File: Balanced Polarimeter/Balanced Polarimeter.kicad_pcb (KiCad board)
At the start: 2 copper layers, 65 x 46.5 mm, 25 parts, among them IC1 OP27, J1 73100-0105, J2 Conn_01x03_Pin, J3 Conn_01x02_Pin, J5 Conn_01x02_Pin, Q1 MMPQ3904, Q2 MMPQ3904, U1 ADA4898-1YRDZ, U2 ADA4898-1YRDZ

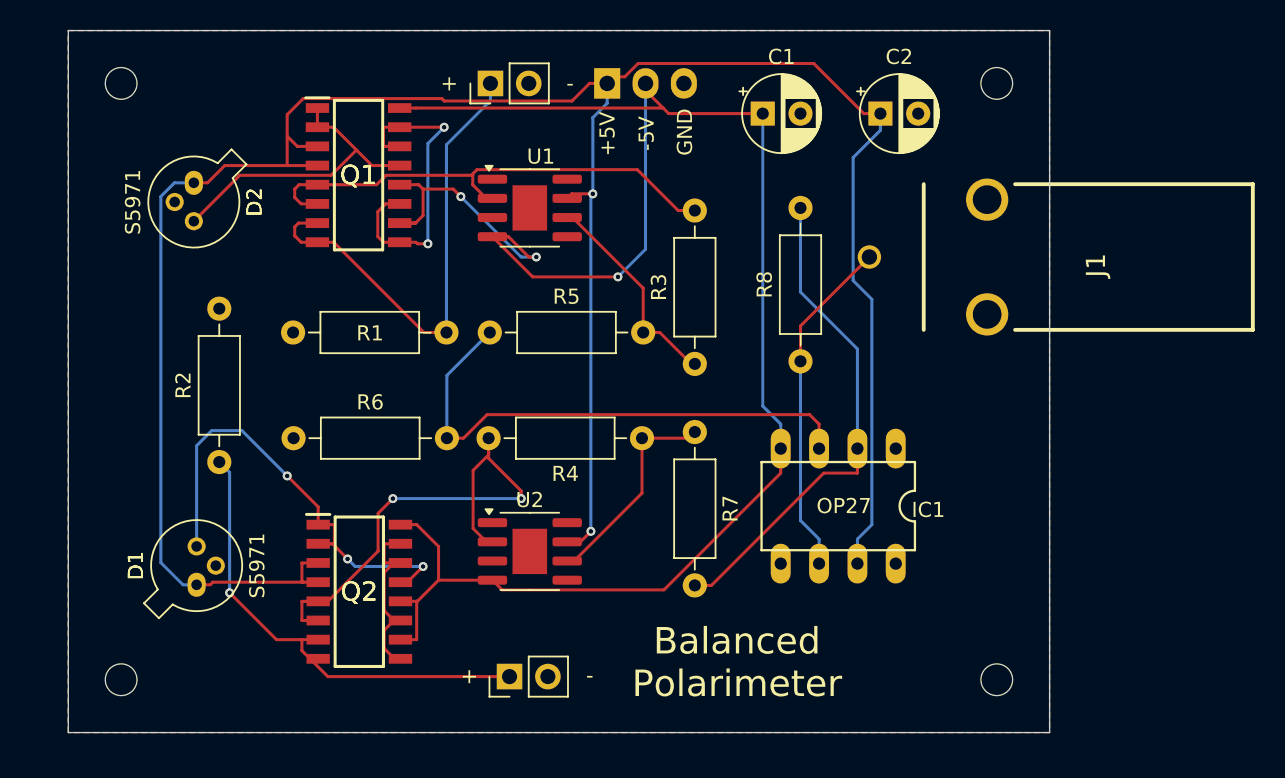
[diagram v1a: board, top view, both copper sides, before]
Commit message: Finalized the PCB Design
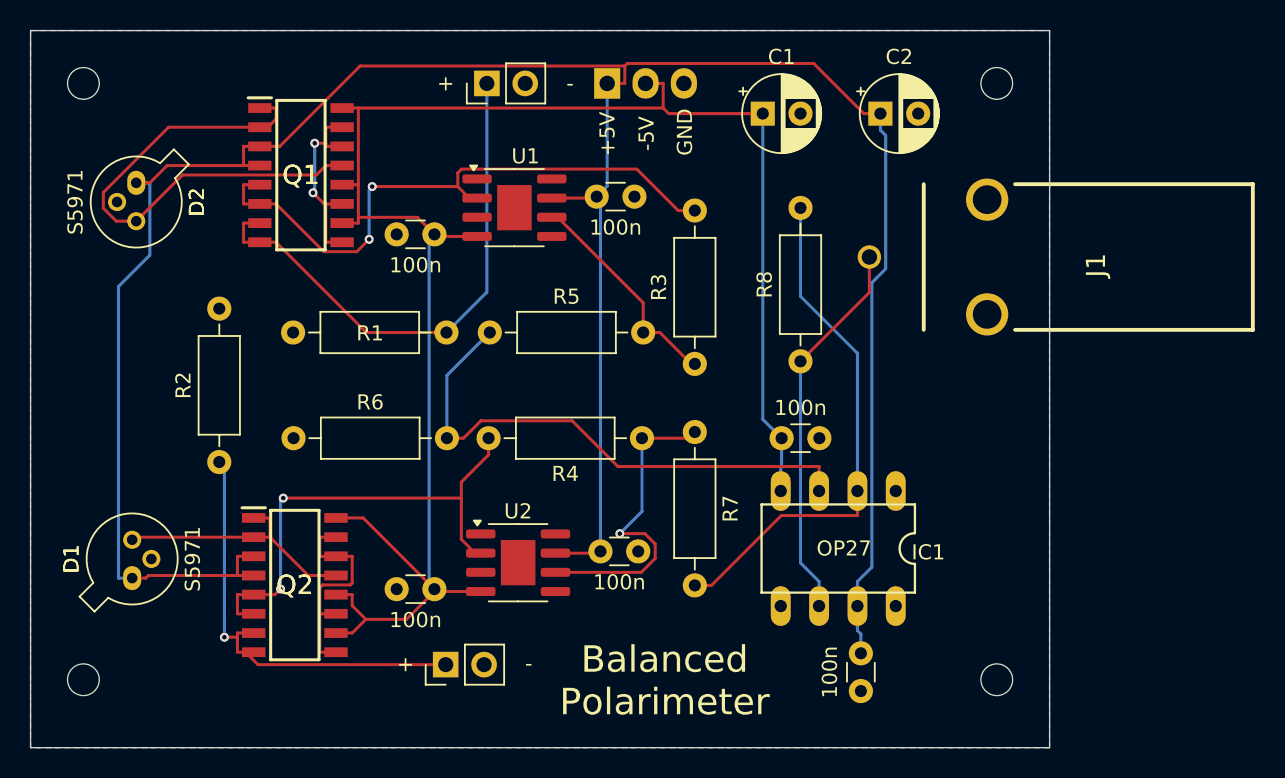
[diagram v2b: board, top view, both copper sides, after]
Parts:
- added C10: 100n, Capacitor_THT:C_Disc_D3.0mm_W1.6mm_P2.50mm, F.Cu at (157.2, 96.0)
- added C11: 100n, Capacitor_THT:C_Disc_D3.0mm_W1.6mm_P2.50mm, F.Cu at (157.0, 72.5)
- added C12: 100n, Capacitor_THT:C_Disc_D3.0mm_W1.6mm_P2.50mm, F.Cu at (143.8, 75.0)
- added C13: 100n, Capacitor_THT:C_Disc_D3.0mm_W1.6mm_P2.50mm, F.Cu at (174.5, 102.8)
- added C14: 100n, Capacitor_THT:C_Disc_D3.0mm_W1.6mm_P2.50mm, F.Cu at (169.2, 88.5)
- added C9: 100n, Capacitor_THT:C_Disc_D3.0mm_W1.6mm_P2.50mm, F.Cu at (143.8, 98.5)
- C1, C2: value C_Polarized -> 1u
- moved J3 4.30 mm to (147.0, 103.5)
- moved Q2 4.29 mm to (137.0, 98.2)
- moved D1 4.29 mm to (126.2, 97.8)
- moved D2 3.82 mm to (126.5, 71.6)
- moved Q1 3.82 mm to (137.4, 71.1)
- moved IC1 2.81 mm to (173.0, 95.8)
- moved H1 2.50 mm to (123.0, 65.0)
- moved H3 2.50 mm to (123.0, 104.5)
- moved U2 1.08 mm to (151.8, 96.8)
- moved U1 1.02 mm to (151.6, 73.2)
- moved J5 0.24 mm to (149.7, 65.0)
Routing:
- net Net-(D1-A): track 31.3 -> 17.0 mm, vias 3 -> 0
- net Net-(D2-A): track 20.8 -> 34.0 mm
- net -5V: track 131.1 -> 120.8 mm, vias 3 -> 0
- net +5V: track 162.1 -> 171.6 mm, vias 2 -> 0
- net Net-(Q1-COLLECTOR_#3_1): track 32.8 -> 41.0 mm, vias 0 -> 2
- net Net-(Q1-BASE_#1): track 21.4 -> 13.3 mm
- net Net-(R4-Pad1): track 14.1 -> 21.2 mm, vias 0 -> 1
- net Net-(J5-Pin_1): track 32.6 -> 35.9 mm
- net V_out: track 22.7 -> 25.5 mm
- net Net-(Q2-BASE_#1): track 12.5 -> 15.0 mm
- net Net-(J3-Pin_1): track 31.8 -> 29.6 mm
- net Net-(Q2-COLLECTOR_#3_1): track 34.1 -> 32.4 mm
- net Net-(IC1-Pad2): track 33.0 -> 34.6 mm
- net Net-(IC1-Pad3): track 35.4 -> 36.2 mm
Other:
- board size 65 x 46.5 mm -> 67.5 x 47.5 mm
